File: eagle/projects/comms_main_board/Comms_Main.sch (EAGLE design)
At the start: 84 parts, among them J1 RECE-20279-001E, Q1 CSD17579Q3A, U1 TPS562209DDCT, U2 LP2985-33DBVR, U3 LP5900TLX-3.3/NOPB, U4 TPS562209DDCT, U5 LMZ34002RKGR, U6 LM3488MMX/NOPB, U7 PCT2075D,118, U8 MS560702BA03-50

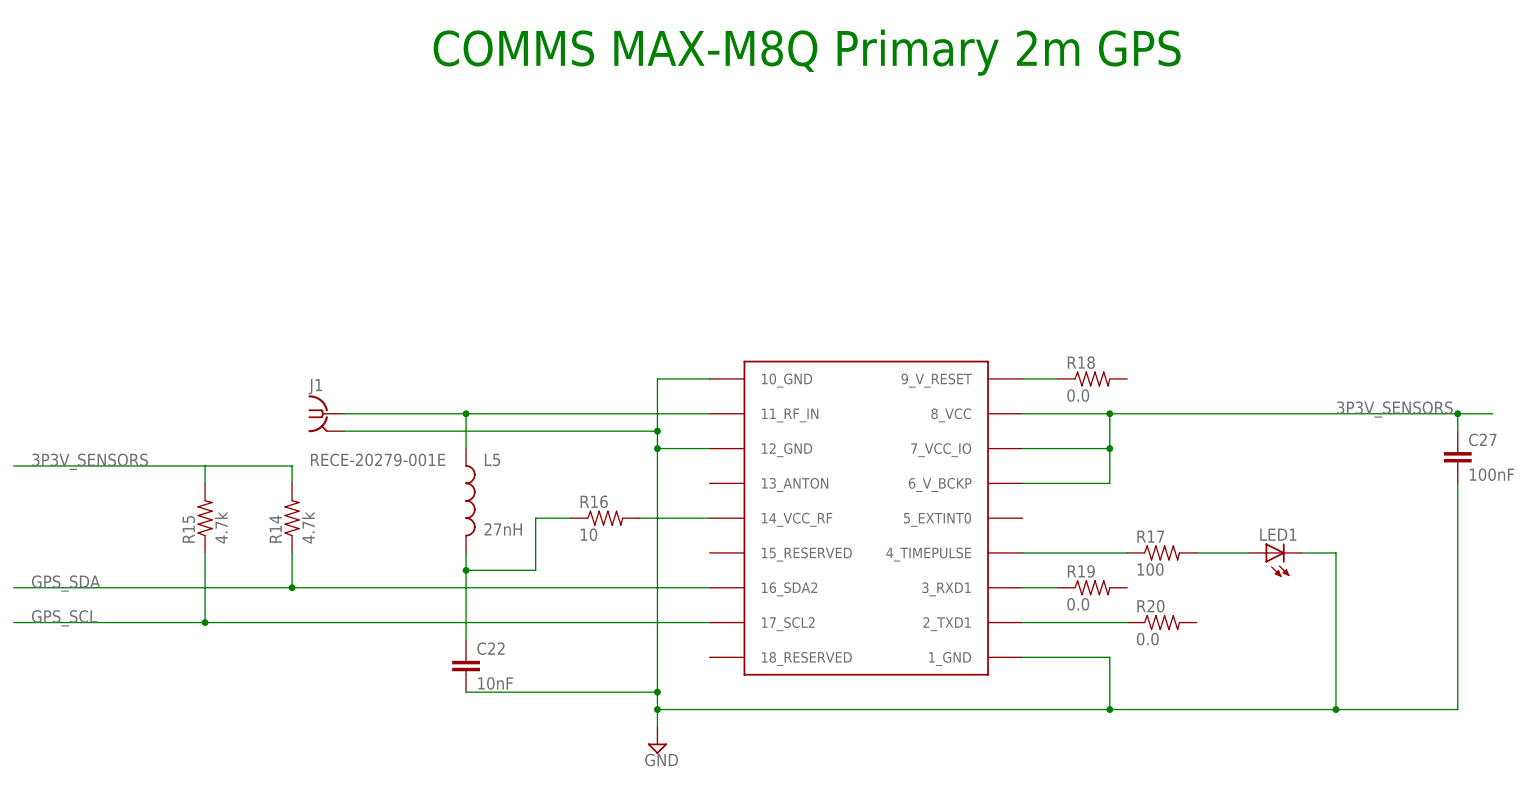
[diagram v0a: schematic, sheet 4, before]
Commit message: Changeess
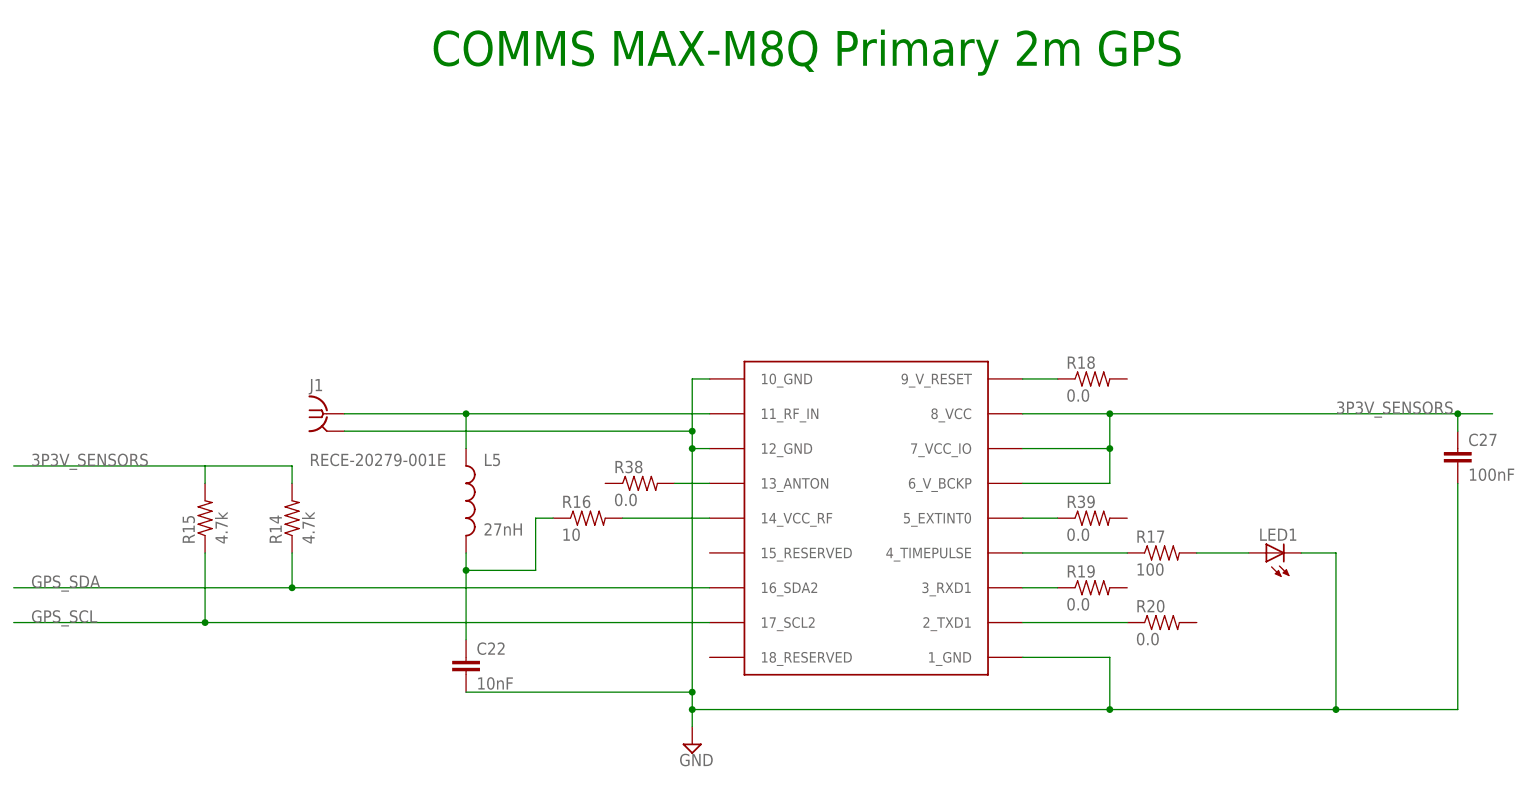
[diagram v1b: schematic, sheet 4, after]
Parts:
- added R38, R39: 0.0, comms:RES_0R0_0805
- renumbered U$1 to U9
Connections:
- new net N$44: R38.2, U9.13_ANTON
- new net N$45: R39.1, U9.5_EXTINT0
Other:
- moved on the sheet: R16
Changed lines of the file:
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@@
 <part name="L4" library="comms" deviceset="L" device="-680ML" technology="_68UH0" value="68uH"/>
 <part name="FRAME4" library="frames" deviceset="A4L-LOC" device=""/>
-<part name="U$1" library="comms" deviceset="UBLOX_MAX" device="" value="MAX-M8Q"/>
 <part name="R14" library="daqcs" deviceset="RES" device="_0603" technology="_4R7" value="4.7k"/>
 <part name="R15" library="daqcs" deviceset="RES" device="_0603" technology="_4R7" value="4.7k"/>
@@
 <part name="R37" library="daqcs" deviceset="RES" device="_0603" technology="_4R7" value="4.7k"/>
 <part name="C27" library="comms" deviceset="CAP" device="_0603" technology="_100NF0" value="100nF"/>
+<part name="R38" library="comms" deviceset="RES" device="_0805" technology="_0R0" value="0.0"/>
+<part name="R39" library="comms" deviceset="RES" device="_0805" technology="_0R0" value="0.0"/>
+<part name="U9" library="comms" deviceset="UBLOX_MAX" device="" value="MAX-M8Q"/>
 </parts>
 <sheets>
@@
 <instances>
 <instance part="FRAME4" gate="G$1" x="0" y="0"/>
-<instance part="U$1" gate="G$1" x="134.62" y="106.68"/>
 <instance part="R14" gate="G$1" x="50.8" y="101.6" rot="R90"/>
 <instance part="R15" gate="G$1" x="38.1" y="101.6" rot="R90"/>
-<instance part="SUPPLY6" gate="GND" x="104.14" y="68.58"/>
+<instance part="SUPPLY6" gate="GND" x="109.22" y="68.58"/>
 <instance part="J1" gate="G$1" x="55.88" y="116.84"/>
-<instance part="R16" gate="G$1" x="96.52" y="101.6"/>
+<instance part="R16" gate="G$1" x="93.98" y="101.6"/>
 <instance part="C22" gate="G$1" x="76.2" y="78.74"/>
 <instance part="L5" gate="G$1" x="76.2" y="104.14"/>
@@
 <instance part="R18" gate="G$1" x="167.64" y="121.92"/>
 <instance part="C27" gate="G$1" x="220.98" y="109.22"/>
+<instance part="R38" gate="G$1" x="101.6" y="106.68"/>
+<instance part="R39" gate="G$1" x="167.64" y="101.6"/>
+<instance part="U9" gate="G$1" x="134.62" y="106.68"/>
 </instances>
 <busses>
@@
 <net name="3P3V_SENSORS" class="0">
 <segment>
-<pinref part="U$1" gate="G$1" pin="8_VCC"/>
 <wire x1="157.48" y1="116.84" x2="170.18" y2="116.84" width="0.1524" layer="91"/>
-<pinref part="U$1" gate="G$1" pin="7_VCC_IO"/>
 <wire x1="157.48" y1="111.76" x2="170.18" y2="111.76" width="0.1524" layer="91"/>
-<pinref part="U$1" gate="G$1" pin="6_V_BCKP"/>
 <wire x1="157.48" y1="106.68" x2="170.18" y2="106.68" width="0.1524" layer="91"/>
 <wire x1="170.18" y1="106.68" x2="170.18" y2="111.76" width="0.1524" layer="91"/>
@@
 <wire x1="220.98" y1="114.3" x2="220.98" y2="116.84" width="0.1524" layer="91"/>
 <junction x="220.98" y="116.84"/>
+<pinref part="U9" gate="G$1" pin="6_V_BCKP"/>
+<pinref part="U9" gate="G$1" pin="7_VCC_IO"/>
+<pinref part="U9" gate="G$1" pin="8_VCC"/>
 </segment>
 <segment>
@@
 <segment>
 <pinref part="SUPPLY6" gate="GND" pin="GND"/>
-<wire x1="104.14" y1="121.92" x2="104.14" y2="114.3" width="0.1524" layer="91"/>
-<wire x1="104.14" y1="114.3" x2="104.14" y2="111.76" width="0.1524" layer="91"/>
-<wire x1="104.14" y1="111.76" x2="104.14" y2="76.2" width="0.1524" layer="91"/>
-<wire x1="104.14" y1="76.2" x2="104.14" y2="73.66" width="0.1524" layer="91"/>
-<wire x1="104.14" y1="73.66" x2="104.14" y2="71.12" width="0.1524" layer="91"/>
-<pinref part="U$1" gate="G$1" pin="12_GND"/>
-<wire x1="111.76" y1="111.76" x2="104.14" y2="111.76" width="0.1524" layer="91"/>
-<junction x="104.14" y="111.76"/>
+<wire x1="109.22" y1="121.92" x2="109.22" y2="114.3" width="0.1524" layer="91"/>
+<wire x1="109.22" y1="114.3" x2="109.22" y2="111.76" width="0.1524" layer="91"/>
+<wire x1="109.22" y1="111.76" x2="109.22" y2="76.2" width="0.1524" layer="91"/>
+<wire x1="109.22" y1="76.2" x2="109.22" y2="73.66" width="0.1524" layer="91"/>
+<wire x1="109.22" y1="73.66" x2="109.22" y2="71.12" width="0.1524" layer="91"/>
+<wire x1="111.76" y1="111.76" x2="109.22" y2="111.76" width="0.1524" layer="91"/>
+<junction x="109.22" y="111.76"/>
 <wire x1="170.18" y1="81.28" x2="170.18" y2="73.66" width="0.1524" layer="91"/>
-<pinref part="U$1" gate="G$1" pin="1_GND"/>
 <wire x1="157.48" y1="81.28" x2="170.18" y2="81.28" width="0.1524" layer="91"/>
-<wire x1="170.18" y1="73.66" x2="104.14" y2="73.66" width="0.1524" layer="91"/>
-<junction x="104.14" y="73.66"/>
-<pinref part="U$1" gate="G$1" pin="10_GND"/>
-<wire x1="111.76" y1="121.92" x2="104.14" y2="121.92" width="0.1524" layer="91"/>
+<wire x1="170.18" y1="73.66" x2="109.22" y2="73.66" width="0.1524" layer="91"/>
+<junction x="109.22" y="73.66"/>
+<wire x1="111.76" y1="121.92" x2="109.22" y2="121.92" width="0.1524" layer="91"/>
 <pinref part="J1" gate="G$1" pin="GND@1"/>
-<wire x1="58.42" y1="114.3" x2="104.14" y2="114.3" width="0.1524" layer="91"/>
-<junction x="104.14" y="114.3"/>
+<wire x1="58.42" y1="114.3" x2="109.22" y2="114.3" width="0.1524" layer="91"/>
+<junction x="109.22" y="114.3"/>
 <pinref part="C22" gate="G$1" pin="2"/>
-<wire x1="76.2" y1="76.2" x2="104.14" y2="76.2" width="0.1524" layer="91"/>
-<junction x="104.14" y="76.2"/>
+<wire x1="76.2" y1="76.2" x2="109.22" y2="76.2" width="0.1524" layer="91"/>
+<junction x="109.22" y="76.2"/>
 <pinref part="LED1" gate="G$1" pin="C"/>
 <wire x1="198.12" y1="96.52" x2="203.2" y2="96.52" width="0.1524" layer="91"/>
@@
 <wire x1="220.98" y1="73.66" x2="203.2" y2="73.66" width="0.1524" layer="91"/>
 <junction x="203.2" y="73.66"/>
+<pinref part="U9" gate="G$1" pin="1_GND"/>
+<pinref part="U9" gate="G$1" pin="10_GND"/>
+<pinref part="U9" gate="G$1" pin="12_GND"/>
 </segment>
 </net>
@@
 <segment>
 <pinref part="J1" gate="G$1" pin="1"/>
-<pinref part="U$1" gate="G$1" pin="11_RF_IN"/>
 <wire x1="58.42" y1="116.84" x2="76.2" y2="116.84" width="0.1524" layer="91"/>
 <pinref part="L5" gate="G$1" pin="1"/>
@@
 <wire x1="76.2" y1="111.76" x2="76.2" y2="116.84" width="0.1524" layer="91"/>
 <junction x="76.2" y="116.84"/>
+<pinref part="U9" gate="G$1" pin="11_RF_IN"/>
 </segment>
 </net>
@@
 <pinref part="R15" gate="G$1" pin="1"/>
 <wire x1="38.1" y1="96.52" x2="38.1" y2="86.36" width="0.1524" layer="91"/>
-<pinref part="U$1" gate="G$1" pin="17_SCL2"/>
 <wire x1="38.1" y1="86.36" x2="111.76" y2="86.36" width="0.1524" layer="91"/>
 <wire x1="38.1" y1="86.36" x2="10.16" y2="86.36" width="0.1524" layer="91"/>
 <junction x="38.1" y="86.36"/>
 <label x="12.7" y="86.36" size="1.778" layer="95"/>
+<pinref part="U9" gate="G$1" pin="17_SCL2"/>
 </segment>
 </net>
 <net name="GPS_SDA" class="0">
 <segment>
-<pinref part="U$1" gate="G$1" pin="16_SDA2"/>
 <wire x1="111.76" y1="91.44" x2="50.8" y2="91.44" width="0.1524" layer="91"/>
 <pinref part="R14" gate="G$1" pin="1"/>
@@
 <junction x="50.8" y="91.44"/>
 <label x="12.7" y="91.44" size="1.778" layer="95"/>
+<pinref part="U9" gate="G$1" pin="16_SDA2"/>
 </segment>
 </net>
 <net name="N$23" class="0">
 <segment>
-<pinref part="U$1" gate="G$1" pin="4_TIMEPULSE"/>
 <pinref part="R17" gate="G$1" pin="1"/>
 <wire x1="157.48" y1="96.52" x2="172.72" y2="96.52" width="0.1524" layer="91"/>
+<pinref part="U9" gate="G$1" pin="4_TIMEPULSE"/>
 </segment>
 </net>
@@
 <net name="N$26" class="0">
 <segment>
-<pinref part="U$1" gate="G$1" pin="3_RXD1"/>
 <wire x1="157.48" y1="91.44" x2="162.56" y2="91.44" width="0.1524" layer="91"/>
 <pinref part="R19" gate="G$1" pin="1"/>
+<pinref part="U9" gate="G$1" pin="3_RXD1"/>
 </segment>
 </net>
 <net name="N$27" class="0">
 <segment>
-<pinref part="U$1" gate="G$1" pin="2_TXD1"/>
 <wire x1="157.48" y1="86.36" x2="172.72" y2="86.36" width="0.1524" layer="91"/>
 <pinref part="R20" gate="G$1" pin="1"/>
+<pinref part="U9" gate="G$1" pin="2_TXD1"/>
 </segment>
 </net>
 <net name="N$28" class="0">
 <segment>
-<pinref part="U$1" gate="G$1" pin="9_V_RESET"/>
 <wire x1="157.48" y1="121.92" x2="162.56" y2="121.92" width="0.1524" layer="91"/>
 <pinref part="R18" gate="G$1" pin="1"/>
+<pinref part="U9" gate="G$1" pin="9_V_RESET"/>
 </segment>
 </net>
 <net name="N$20" class="0">
 <segment>
-<pinref part="U$1" gate="G$1" pin="14_VCC_RF"/>
 <pinref part="R16" gate="G$1" pin="2"/>
-<wire x1="111.76" y1="101.6" x2="101.6" y2="101.6" width="0.1524" layer="91"/>
+<wire x1="111.76" y1="101.6" x2="99.06" y2="101.6" width="0.1524" layer="91"/>
+<pinref part="U9" gate="G$1" pin="14_VCC_RF"/>
 </segment>
 </net>
@@
 <pinref part="R16" gate="G$1" pin="1"/>
 <wire x1="76.2" y1="93.98" x2="76.2" y2="96.52" width="0.1524" layer="91"/>
-<wire x1="91.44" y1="101.6" x2="86.36" y2="101.6" width="0.1524" layer="91"/>
+<wire x1="88.9" y1="101.6" x2="86.36" y2="101.6" width="0.1524" layer="91"/>
 <wire x1="86.36" y1="101.6" x2="86.36" y2="93.98" width="0.1524" layer="91"/>
 <wire x1="86.36" y1="93.98" x2="76.2" y2="93.98" width="0.1524" layer="91"/>
@@
 </segment>
 </net>
+<net name="N$44" class="0">
+<segment>
+<pinref part="R38" gate="G$1" pin="2"/>
+<wire x1="106.68" y1="106.68" x2="111.76" y2="106.68" width="0.1524" layer="91"/>
+<pinref part="U9" gate="G$1" pin="13_ANTON"/>
+</segment>
+</net>
+<net name="N$45" class="0">
+<segment>
+<pinref part="R39" gate="G$1" pin="1"/>
+<wire x1="157.48" y1="101.6" x2="162.56" y2="101.6" width="0.1524" layer="91"/>
+<pinref part="U9" gate="G$1" pin="5_EXTINT0"/>
+</segment>
+</net>
